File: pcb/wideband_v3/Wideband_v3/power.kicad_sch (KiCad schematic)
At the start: 24 parts, among them Q1 SS8050, Q2 IRLZ44N, Q3 IRLZ44N, U5 LT4363IMS, U6 TPS5430DDA

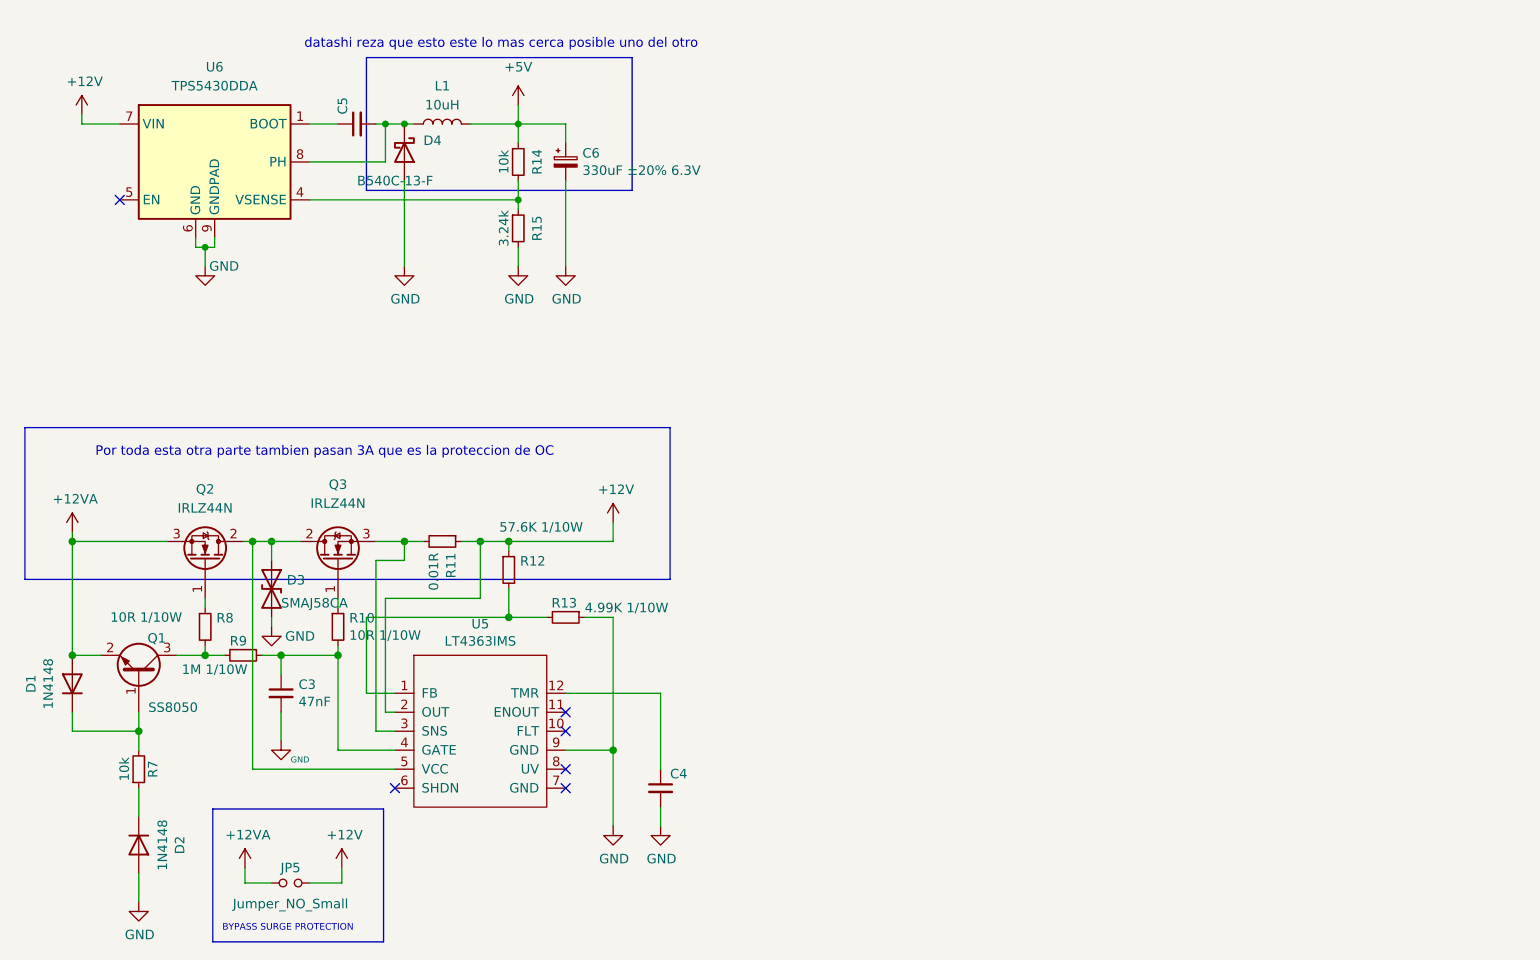
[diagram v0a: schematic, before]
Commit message: init 7seg pcb
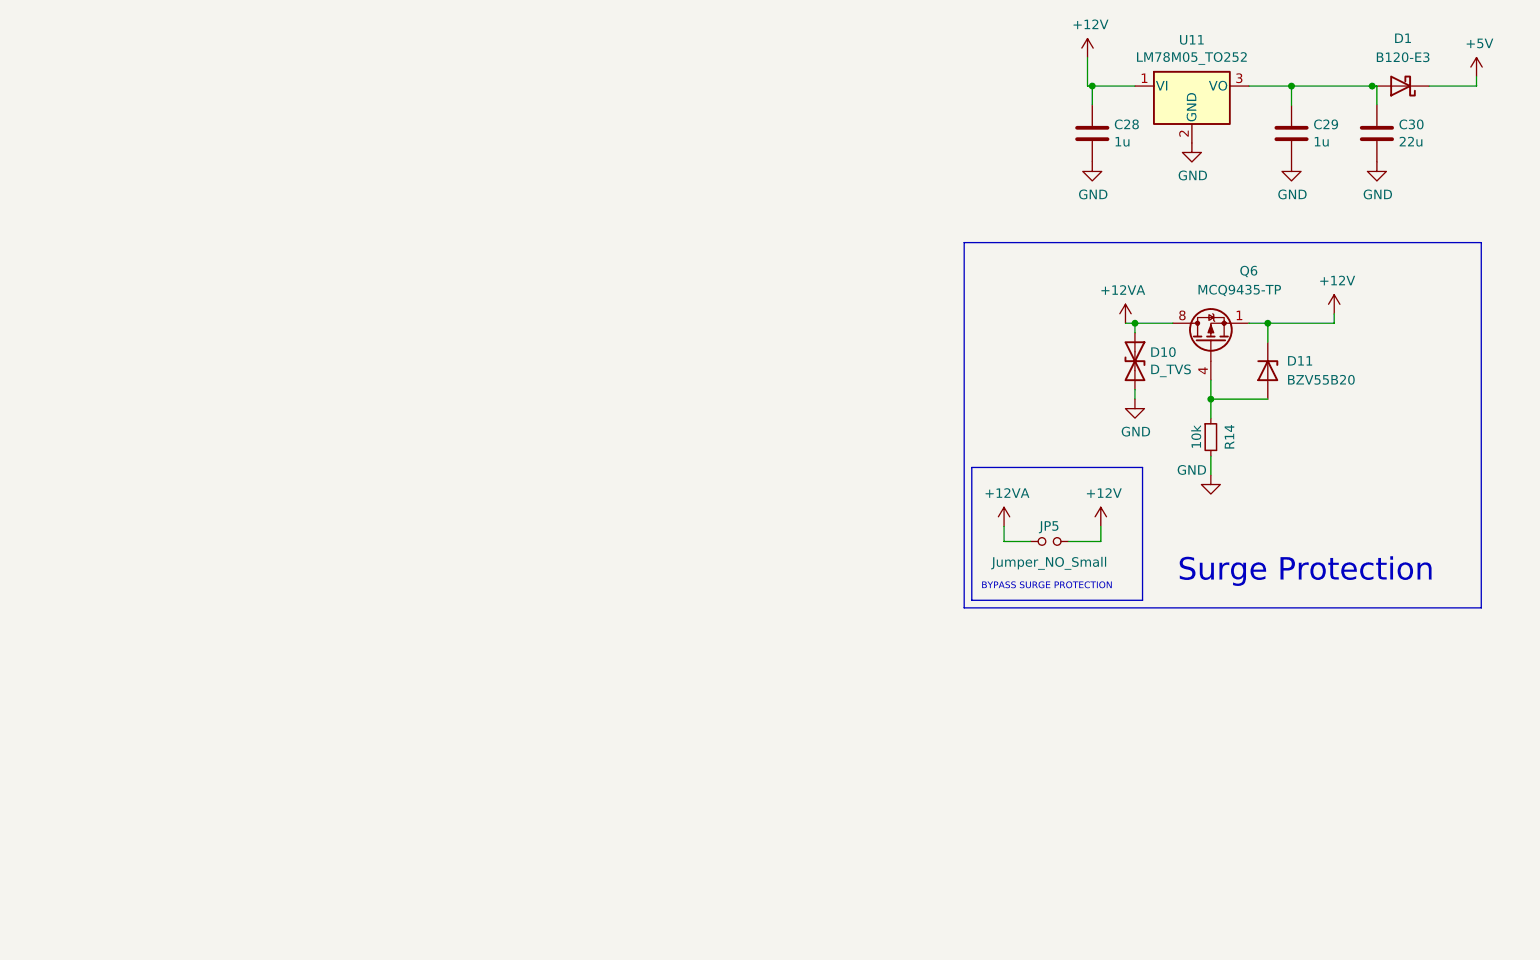
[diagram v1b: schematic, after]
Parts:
- removed C3: 47nF, Capacitor_SMD:C_0603_1608Metric, symbol Device:C_Small
- removed C4: 100nF, Capacitor_SMD:C_0805_2012Metric, symbol Device:C_Small
- removed C5: 10nF, Capacitor_SMD:C_0805_2012Metric, symbol Device:C_Small
- removed C6: 330uF ±20% 6.3V, Capacitor_SMD:CP_Elec_6.3x7.7, symbol Device:CP_Small
- removed D1, D2: 1N4148, Diode_SMD:D_SOD-523, symbol Diode:1N4148
- removed D3: SMAJ58CA, Diode_SMD:D_SMA, symbol Device:D_TVS
- removed D4: B540C-13-F, Diode_SMD:D_SMA, symbol Device:D_Schottky
- removed L1: 10uH, Inductor_SMD:L_7.3x7.3_H4.5, symbol Device:L
- removed Q1: SS8050, Package_TO_SOT_SMD:SOT-23, symbol Transistor_BJT:2N3055
- removed Q2, Q3: IRLZ44N, Package_TO_SOT_SMD:TO-252-2, symbol Transistor_FET:IRLZ44N
- removed R10, R8: 10R 1/10W, Resistor_SMD:R_0603_1608Metric, symbol Device:R_Small
- removed R11: 0.01R, Resistor_SMD:R_1210_3225Metric, symbol Device:R_Small
- removed R12: 57.6K 1/10W, Resistor_SMD:R_0603_1608Metric, symbol Device:R_Small
- removed R13: 4.99K 1/10W, Resistor_SMD:R_0603_1608Metric, symbol Device:R_Small
- removed R15: 3.24k, Resistor_SMD:R_0603_1608Metric, symbol Device:R_Small
- removed R7: 10k, Resistor_SMD:R_0805_2012Metric, symbol Device:R_Small
- removed R9: 1M 1/10W, Resistor_SMD:R_0603_1608Metric, symbol Device:R_Small
- removed U5: LT4363IMS, Package_SO:MSOP-12_3x4mm_P0.65mm, symbol OpenEFI-STM32-rev3:LT4363IMS
- removed U6: TPS5430DDA, Package_SO:TI_SO-PowerPAD-8_ThermalVias, symbol Regulator_Switching:TPS5430DDA
- added C28, C29: 1u, Capacitor_SMD:C_0603_1608Metric, symbol Device:C
- added C30: 22u, Capacitor_SMD:C_0805_2012Metric, symbol Device:C
- added D1: B120-E3, Diode_SMD:D_SMA, symbol Diode:B120-E3
- added D10: D_TVS, Diode_SMD:D_SMC, symbol Device:D_TVS
- added D11: BZV55B20, Diode_SMD:D_MiniMELF, symbol Diode:BZV55B20
- added Q6: MCQ9435-TP, Package_SO:SOIC-8_3.9x4.9mm_P1.27mm, symbol Transistor_FET:IRF7404
- added U11: LM78M05_TO252, Package_TO_SOT_SMD:TO-252-2, symbol Regulator_Linear:LM78M05_TO252
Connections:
- net +12V: now also C28.1, D11.1 (K), Q6.1 (S), Q6.2 (S), Q6.3 (S), U11.1 (VI)
- net +12VA: now also D10.1 (A1), Q6.5 (D), Q6.6 (D), Q6.7 (D), Q6.8 (D)
- net +5V: now also D1.1 (K); no longer R14.1
- net GND: now also R14.2, C28.2, C29.2, C30.2, D10.2 (A2), U11.2 (GND)
- new net: C29.1, C30.1, D1.2 (A), U11.3 (VO)
- new net: D11.2 (A), Q6.4 (G), R14.1
- no-connect marks 6 -> 0
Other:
- note added: "Surge Protection"
- note removed: "Por toda esta otra parte tambien pasan 3A que es la proteccion de OC"
- note removed: "datashi reza que esto este lo mas cerca posible uno del otro"
- moved on the sheet: JP5
